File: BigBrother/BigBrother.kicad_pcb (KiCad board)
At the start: 2 copper layers, 4 parts, among them J1 RPi_GPIO, U1 bno055, U2 BMP388, U3 VHN5019_Breakout

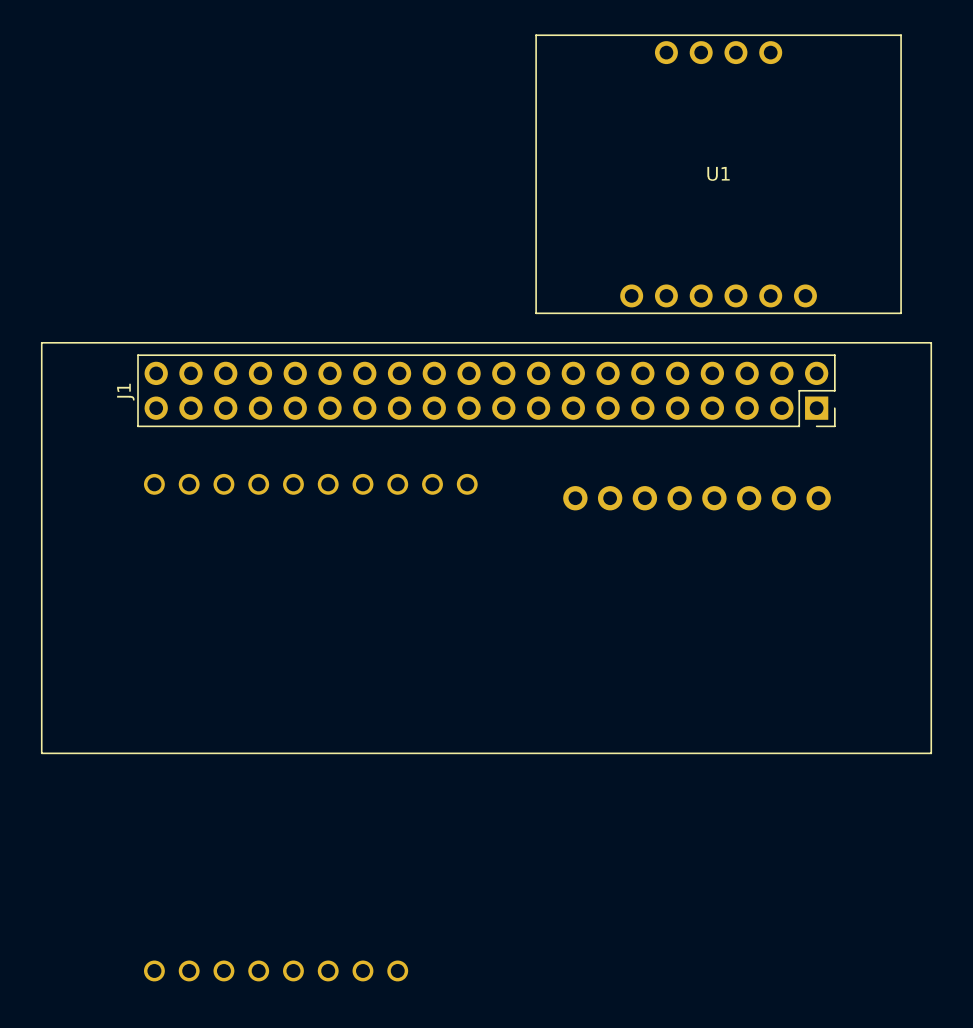
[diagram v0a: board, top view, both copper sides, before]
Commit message: Board!! maybe done!!!
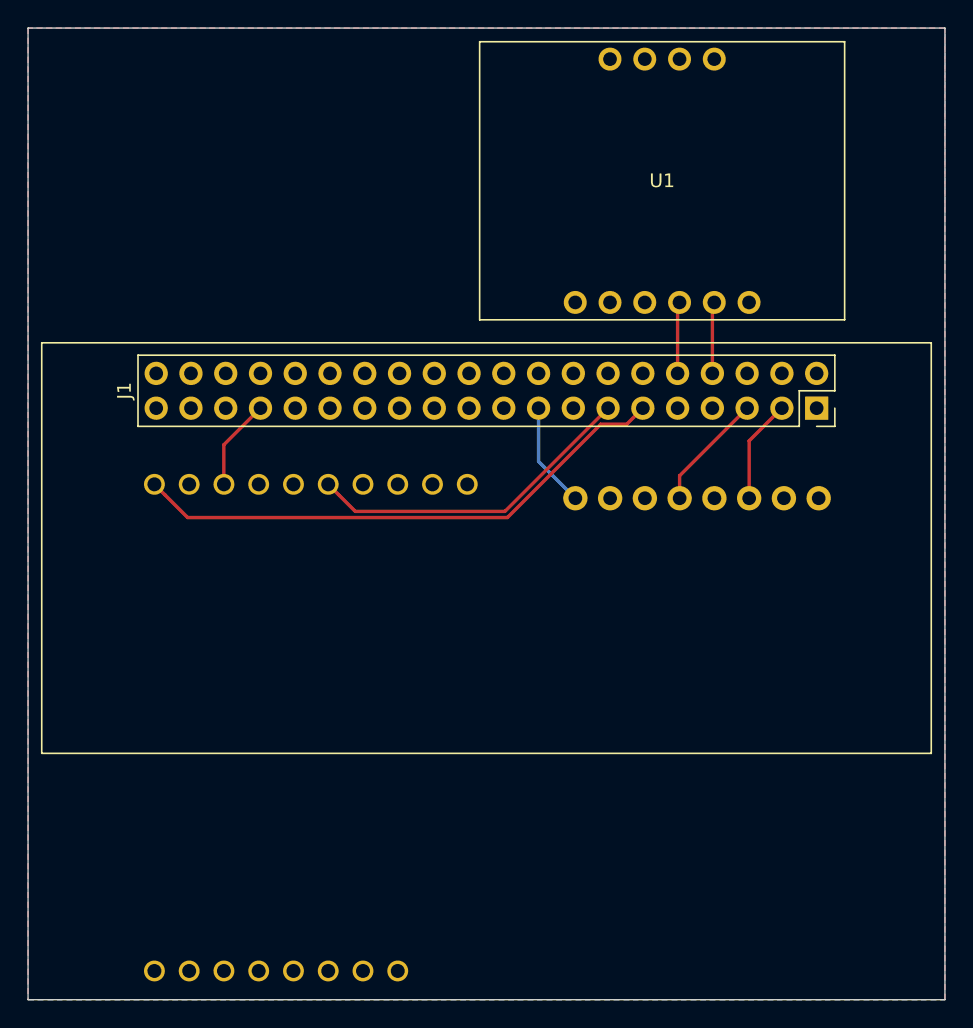
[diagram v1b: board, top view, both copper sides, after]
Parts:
- moved U1 4.15 mm to (145.0, 56.0)
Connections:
- J1 pad 1: Net-(J1-Pad1) -> 3.3V
- J1 pad 14: Net-(J1-Pad14) -> GND
- J1 pad 20: GND2 -> GND
- J1 pad 25: Net-(J1-Pad25) -> GND
- J1 pad 30: Net-(J1-Pad30) -> GND
- J1 pad 34: Net-(J1-Pad34) -> GND
- J1 pad 39: Net-(J1-Pad39) -> GND
- J1 pad 6: Net-(J1-Pad6) -> GND
- U3 pad 8: GND2 -> GND
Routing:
- net GPIO_INA: track 0.00 -> 40.0 mm
- net GPIO_INB: track 0.00 -> 24.4 mm
- net SCL: track 0.00 -> 8.62 mm
- net 3.3V: track 0.00 -> 7.70 mm
- net SDA: track 0.00 -> 7.57 mm
- net GPIO_PWM: track 0.00 -> 6.67 mm
- net TXD: track 0.00 -> 5.24 mm
- net RXD: track 0.00 -> 5.24 mm
- added copper zone on F.Cu, net 3.3V
- added copper zone on B.Cu, net GND
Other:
- board outline added: 67 x 71 mm
